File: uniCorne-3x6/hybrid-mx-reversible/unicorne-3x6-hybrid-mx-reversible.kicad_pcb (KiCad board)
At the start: 2 copper layers, 133.8 x 91.4 mm, 98 parts, among them J1 MJ-4PP-9, J2 Nice!View, J3 Conn_01x02, J4 Conn_01x03, SW1 SW_MX_HS, SW10 SW_MX_HS, SW11 SW_MX_HS, SW12 SW_MX_HS, SW13 SW_MX_HS, SW14 SW_MX_HS, SW15 SW_MX_HS, SW16 SW_MX_HS, SW17 SW_MX_HS, SW18 SW_MX_HS, SW19 SW_CHOC_HS, SW2 SW_MX_HS, SW20 SW_CHOC_HS, SW21 SW_CHOC_HS, SW3 SW_MX_HS, SW4 SW_MX_HS, SW5 SW_MX_HS, SW6 SW_MX_HS, SW7 SW_MX_HS, SW8 SW_MX_HS, SW9 SW_MX_HS, U1 ProMicro-ish

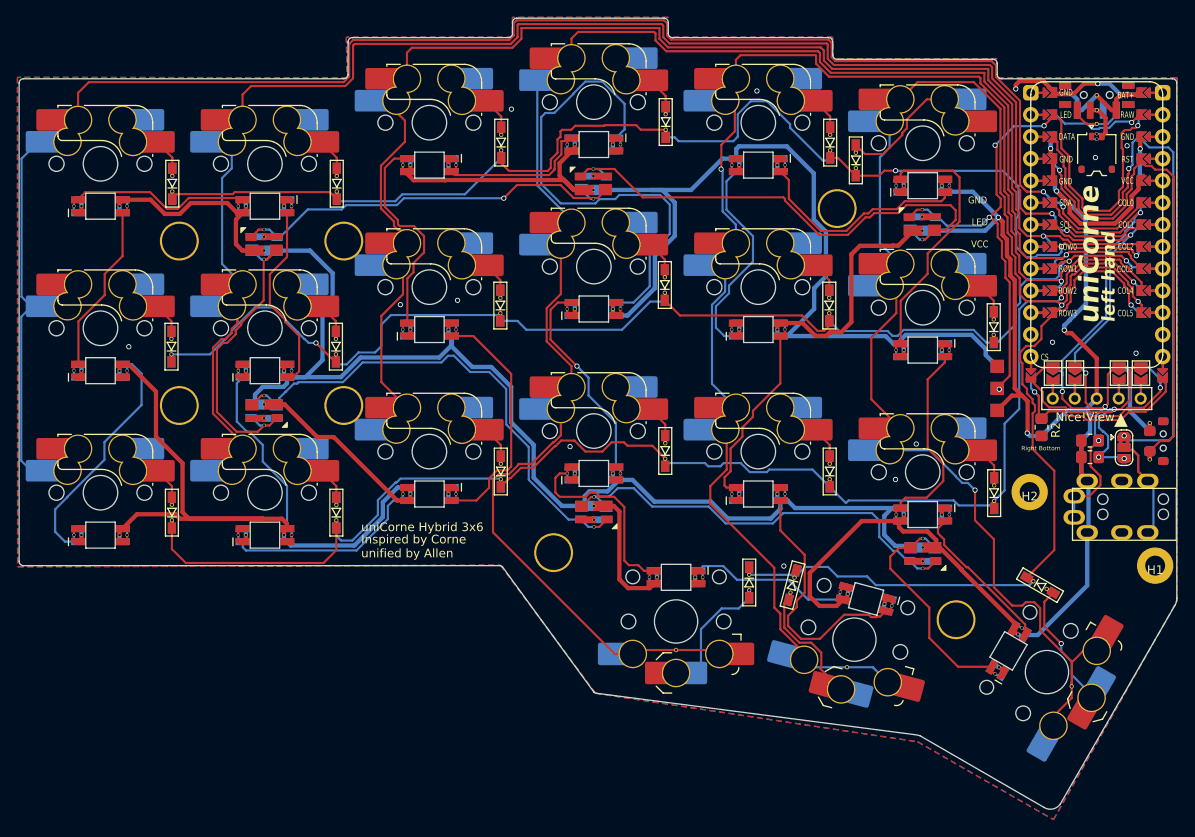
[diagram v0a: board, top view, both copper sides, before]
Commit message: small tweak
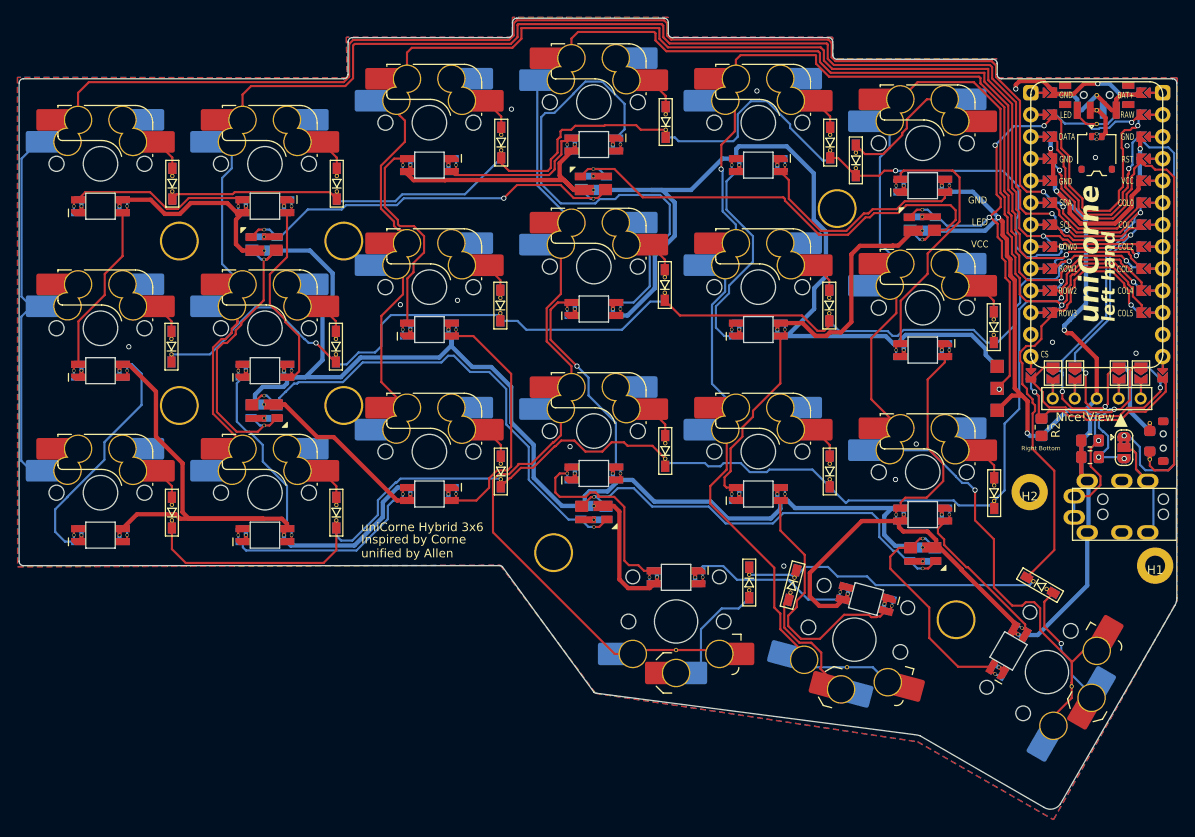
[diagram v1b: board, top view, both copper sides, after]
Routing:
- net col0: track 197.3 -> 192.3 mm
- net DATA: track 67.7 -> 72.4 mm
- net RESET: track 59.1 -> 62.9 mm
- net SDA: track 66.5 -> 63.9 mm
- net SCL: track 58.7 -> 56.8 mm
- net col1: track 170.8 -> 169.2 mm
- net unconnected-(PSW1-C-Pad3): track 6.50 -> 5.34 mm
- net col5: track 153.3 -> 152.2 mm, vias 3 -> 2
- net VCC: track 584.3 -> 583.3 mm
- net GND: track 36.9 -> 35.9 mm
- net row2: track 159.0 -> 158.2 mm
- net row3: track 87.1 -> 86.6 mm
